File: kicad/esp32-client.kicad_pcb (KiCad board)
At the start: 2 copper layers, 36 x 56 mm, 42 parts, among them J1 Conn_01x01_Pin, J2 Conn_01x01_Pin, J3 Conn_01x02, P1 USB_C_Plug_USB2.0, Q1 BCW66G, Q2 BCW66G, U1 ESP32-C3-MINI-1, U2 DRV8833PW, U3 TP4056-42-ESOP8, U4 U8205A, U5 DW01A, U6 USBLC6-2P6, U7 CH340C, U8 AMS1117-3.3

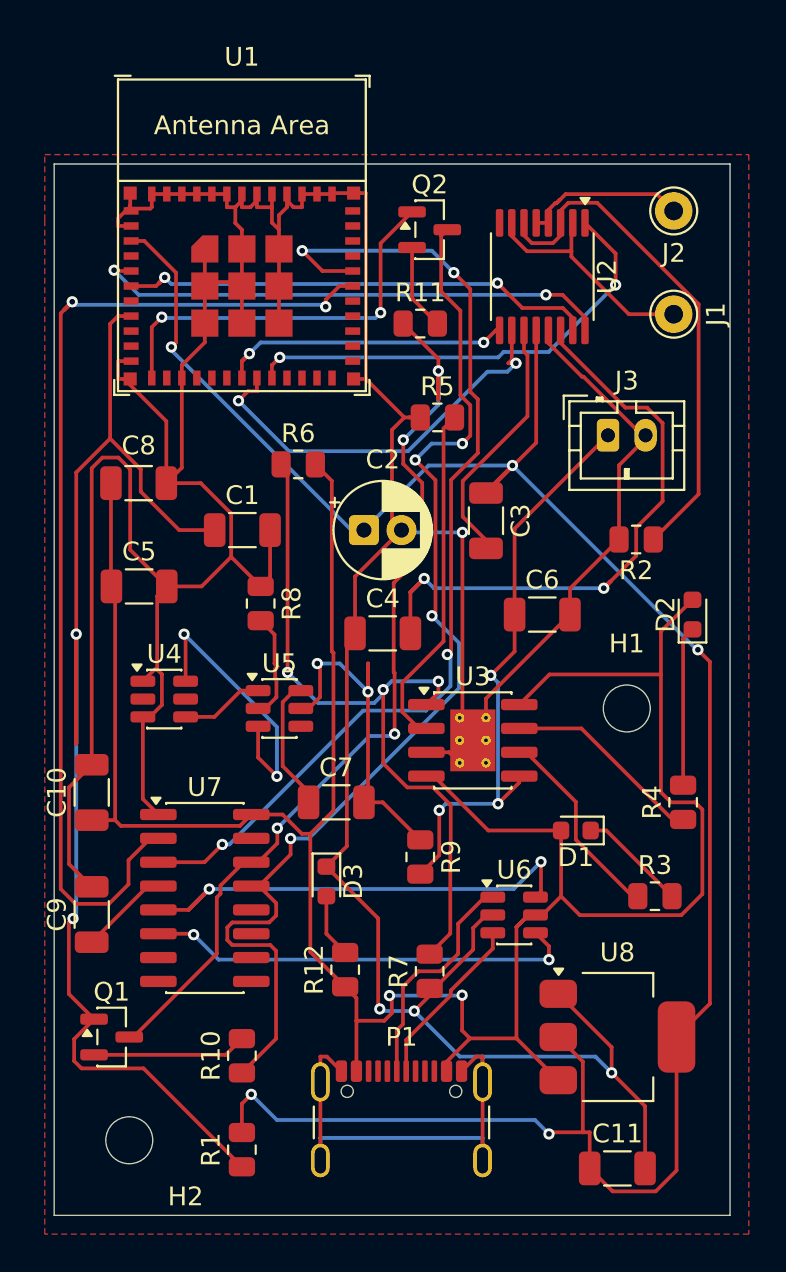
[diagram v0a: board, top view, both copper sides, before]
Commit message: init
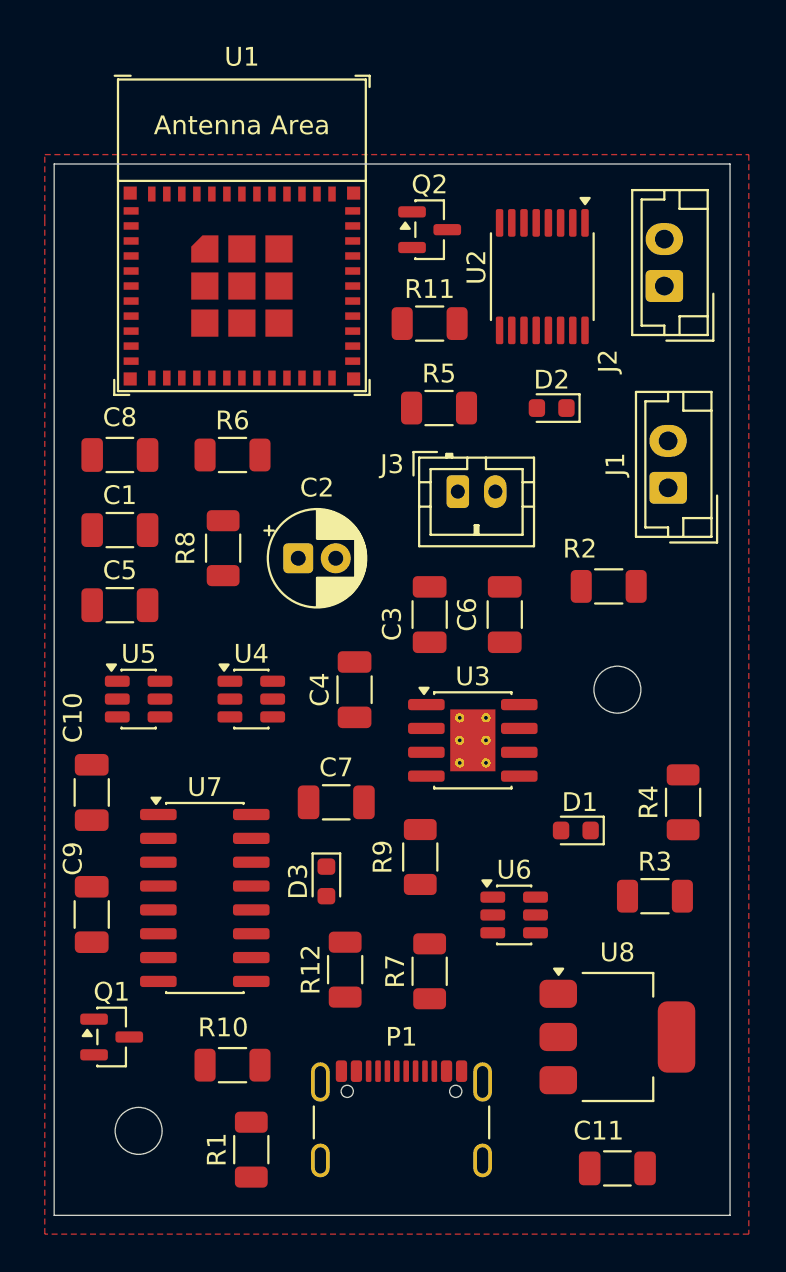
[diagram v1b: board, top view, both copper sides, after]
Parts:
- J1, J2: value Conn_01x01_Pin -> Conn_01x02; footprint Connector_Pin:Pin_D1.0mm_L10.0mm -> Connector_JST:JST_EH_B2B-EH-A_1x02_P2.50mm_Vertical
- R1, R10, R11, R12, R2, R3, R4, R5, R6, R7, R8, R9: footprint Resistor_SMD:R_0805_2012Metric -> Resistor_SMD:R_1206_3216Metric
- moved D2 13.3 mm to (197.0, 67.5), turned to 180 degrees
- moved J1 9.25 mm to (203.2, 71.8)
- moved J3 8.54 mm to (192.0, 72.0)
- moved U5 7.52 mm to (175.0, 83.0)
- moved C1 6.53 mm to (174.0, 74.0)
- moved C3 5.83 mm to (190.5, 78.5)
- moved U4 4.64 mm to (181.0, 83.0)
- moved J2 4.03 mm to (203.0, 61.0), turned to 90 degrees
- moved C2 3.81 mm to (183.5, 75.5)
- moved R8 3.56 mm to (179.5, 75.0)
- moved R6 3.54 mm to (180.0, 70.0)
- moved C4 3.35 mm to (186.5, 82.5), turned to 90 degrees
- moved R2 2.90 mm to (200.0, 77.0), turned to 0 degrees
- moved C6 2.00 mm to (194.5, 78.5), turned to 90 degrees
- moved C8 1.80 mm to (174.0, 70.0)
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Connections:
- U2 pad 4: Net-(J2-Pin_1) -> Net-(J1-Pin_2)
- U2 pad 5: Net-(J2-Pin_1) -> Net-(J2-Pin_2)
- U2 pad 7: Net-(J1-Pin_1) -> Net-(J2-Pin_1)
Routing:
- net GND: track 278.4 -> 0.00 mm, vias 4 -> 0
- net +5V: track 138.9 -> 0.00 mm, vias 2 -> 0
- net +3.3V: track 119.7 -> 0.00 mm, vias 5 -> 0
- net /power/EN: track 86.6 -> 0.00 mm, vias 2 -> 0
- net Net-(Q2-E): track 61.3 -> 0.00 mm, vias 4 -> 0
- net /power/TXD: track 57.5 -> 0.00 mm, vias 2 -> 0
- net /power/RXD: track 55.1 -> 0.00 mm, vias 4 -> 0
- net Net-(Q1-E): track 54.3 -> 0.00 mm, vias 4 -> 0
- net Net-(U3-TEMP): track 38.9 -> 0.00 mm, vias 3 -> 0
- net Net-(U2-VINT): track 37.3 -> 0.00 mm, vias 2 -> 0
- net Net-(J3-Pin_1): track 31.4 -> 0.00 mm, vias 3 -> 0
- net Net-(U7-UD+): track 29.7 -> 0.00 mm, vias 2 -> 0
- net /motor_driver/AN_1_PWM: track 27.7 -> 0.00 mm, vias 2 -> 0
- net Net-(U2-AISEN): track 27.6 -> 0.00 mm
- net /motor_driver/AN_2_DIR: track 27.2 -> 0.00 mm, vias 2 -> 0
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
